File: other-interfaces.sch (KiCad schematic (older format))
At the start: 24 parts, among them J5 DM3AT-SF-PEJM5, J7 BM04B-SRSS-TB-LF-SN, U23 NTS0102GT

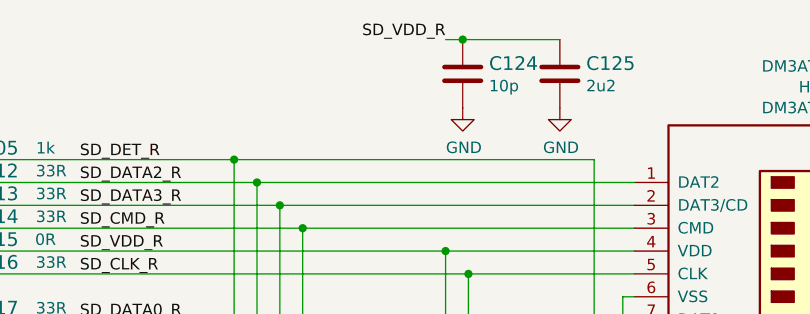
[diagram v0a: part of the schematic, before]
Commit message: Cleanup
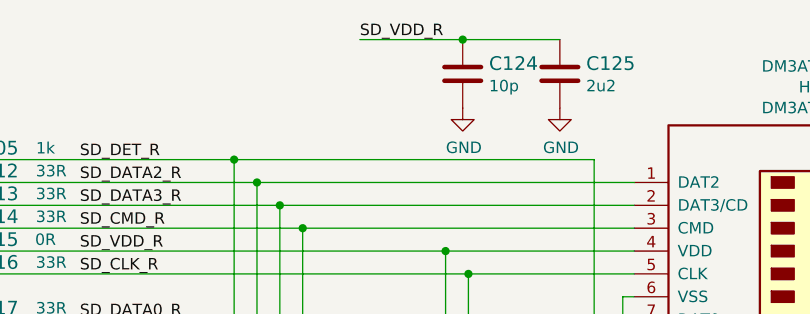
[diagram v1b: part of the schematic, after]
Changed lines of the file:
@@
 $Descr A4 11693 8268
 encoding utf-8
-Sheet 9 13
+Sheet 9 12
 Title ""
 Date ""
@@
 Wire Wire Line
 	2700 2600 2700 2675
-Text Label 5075 2150 2    50   ~ 0
+Text Label 4700 2150 0    50   ~ 0
 SD_VDD_R
 $Comp
@@
 $EndComp
 Wire Wire Line
-	5075 2150 5150 2150
+	4700 2150 5150 2150
 $Comp
 L sa800u-baseboard-hw:C_10p_0402 C124
